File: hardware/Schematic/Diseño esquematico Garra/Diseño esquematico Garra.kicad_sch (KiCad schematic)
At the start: 12 parts, among them J1 Screw_Terminal_01x02

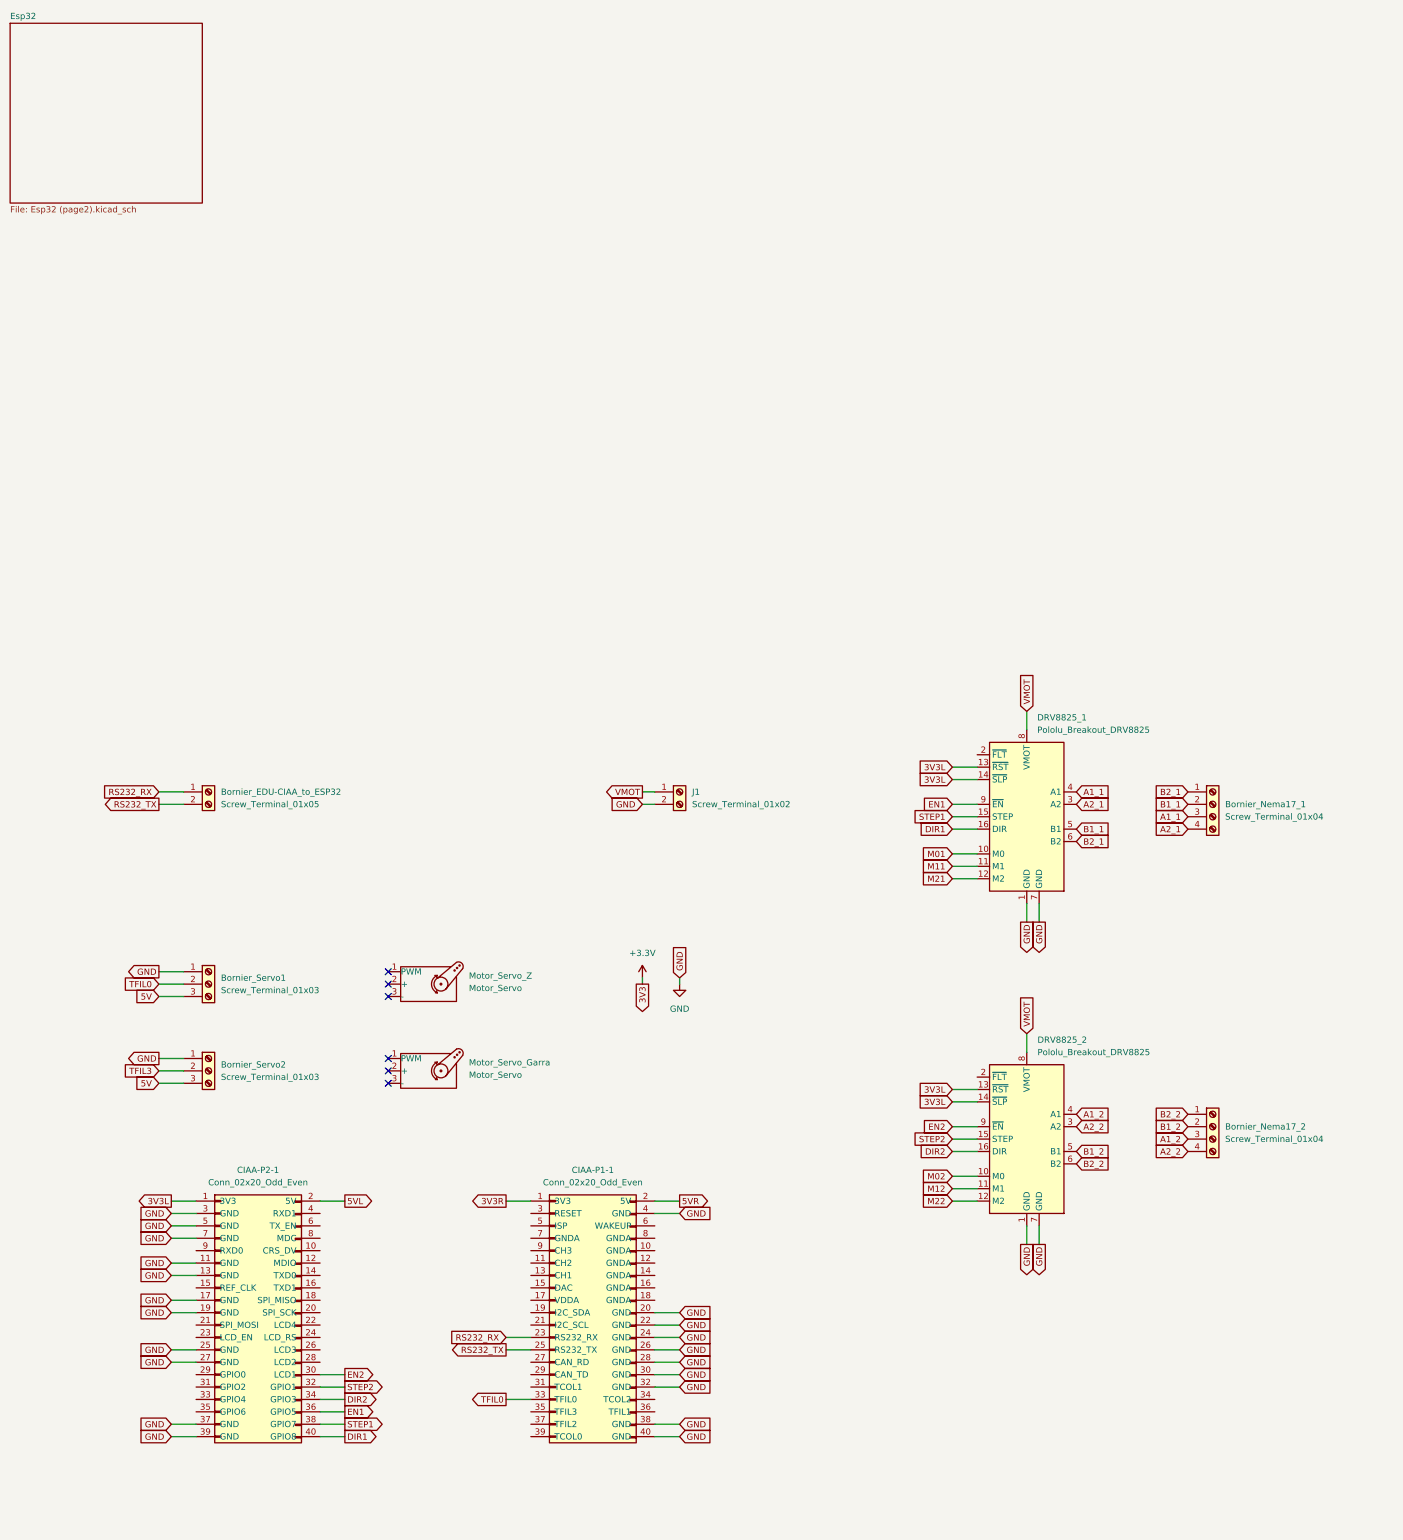
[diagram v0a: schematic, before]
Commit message: Schematics updated + PCB
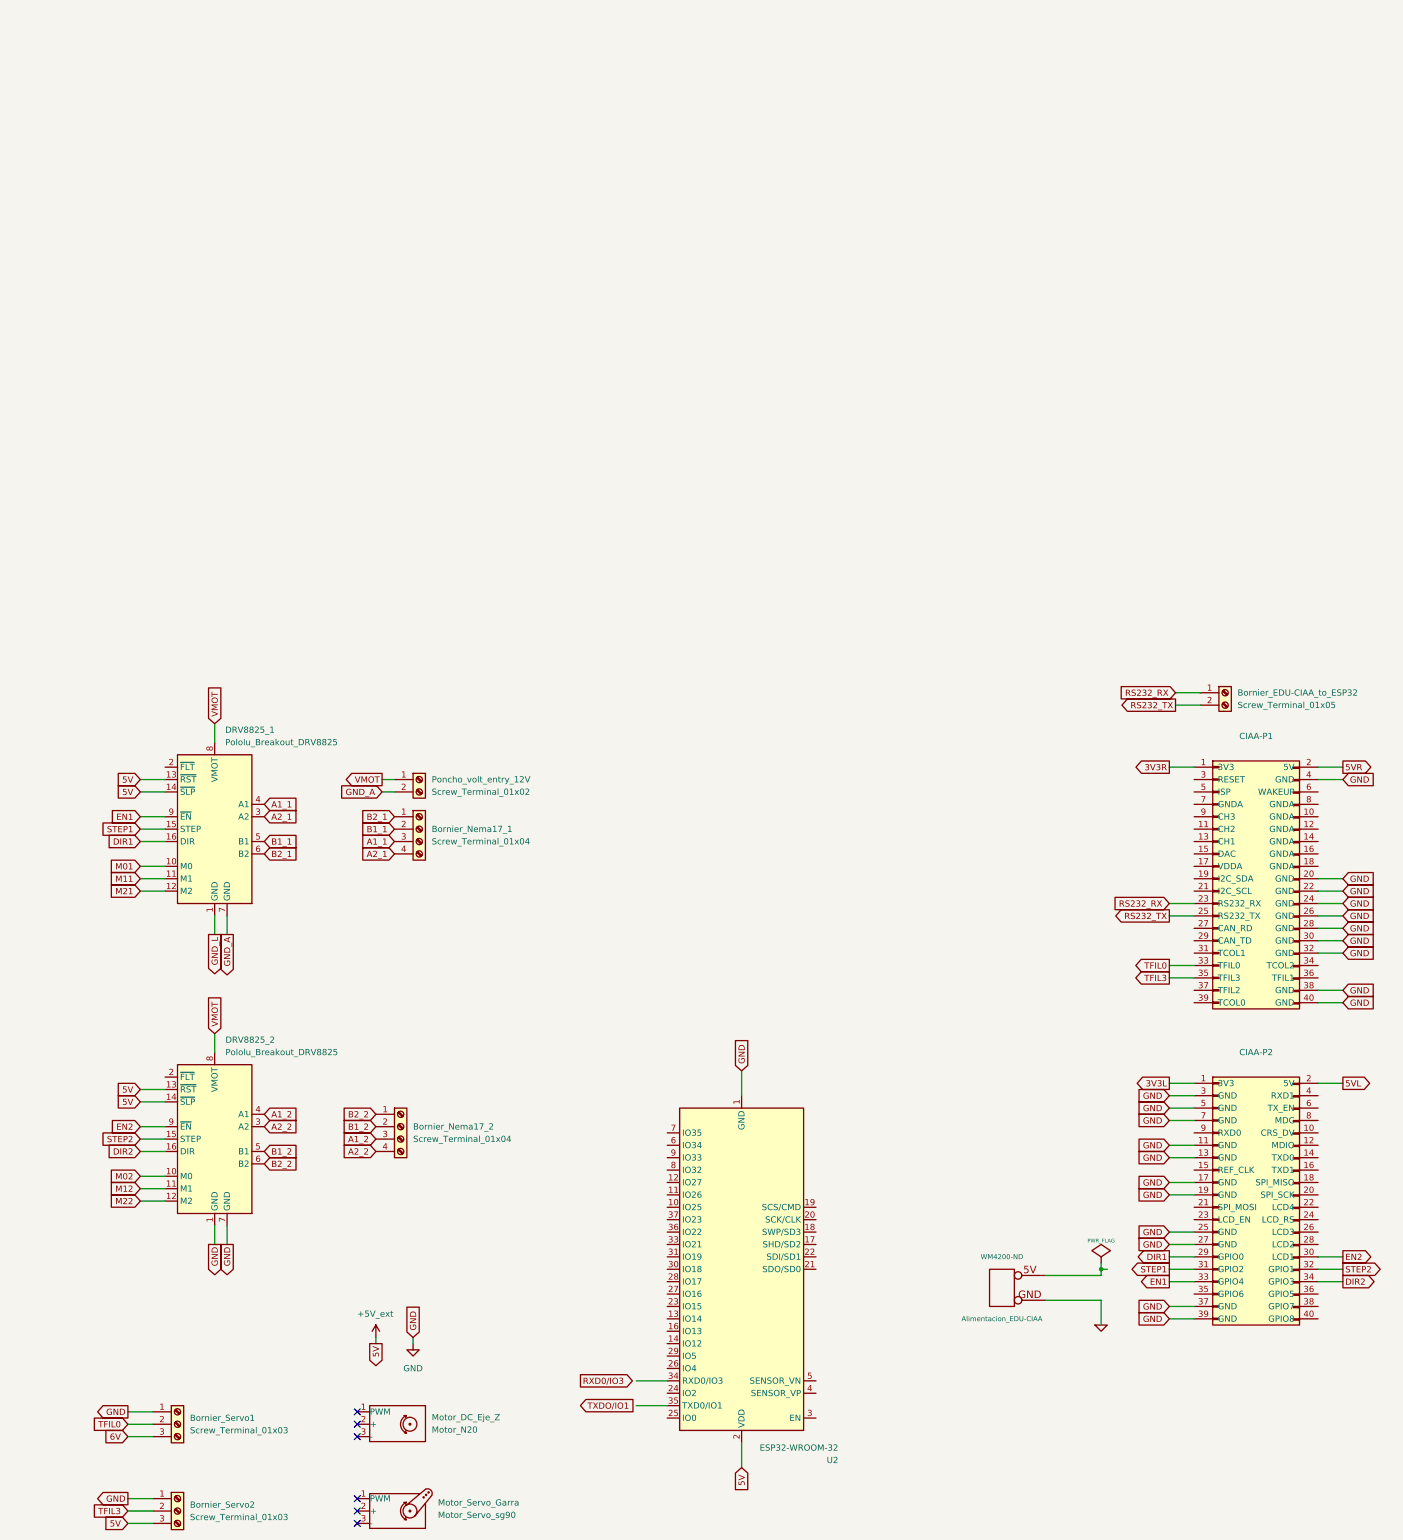
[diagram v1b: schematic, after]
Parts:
- added Alimentacion_EDU-CIAA: WM4200-ND, ~, symbol edu-ciaa-nxp:CONN_2
- added U2: ESP32-WROOM-32, RF_Module:ESP32-WROOM-32, symbol RF_Module:ESP32-WROOM-32
- CIAA-P1: renamed from CIAA-P1-1; value Conn_02x20_Odd_Even -> ~
- CIAA-P2: renamed from CIAA-P2-1; value Conn_02x20_Odd_Even -> ~
- Motor_DC_Eje_Z: renamed from Motor_Servo_Z; value Motor_Servo -> Motor_N20
- Motor_Servo_Garra: value Motor_Servo -> Motor_Servo_sg90
- renumbered J1 to Poncho_volt_entry_12V
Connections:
- net 3V3L: no longer DRV8825_1.13 (~{RST}), DRV8825_1.14 (~{SLP}), DRV8825_2.13 (~{RST}), DRV8825_2.14 (~{SLP})
- net DIR1: now also CIAA-P2.29 (GPIO0); no longer CIAA-P2.40 (GPIO8)
- net EN1: now also CIAA-P2.33 (GPIO4); no longer CIAA-P2.36 (GPIO5)
- net GND: now also Alimentacion_EDU-CIAA.GND (P1), U2.1 (GND), U2.15 (GND), U2.38 (GND), U2.39 (GND); no longer DRV8825_1.1 (GND), DRV8825_1.7 (GND), Poncho_volt_entry_12V.2 (Pin_2)
- net STEP1: now also CIAA-P2.31 (GPIO2); no longer CIAA-P2.38 (GPIO7)
- net TFIL3: now also CIAA-P1.35 (TFIL3)
- net 5V renamed +5V_ext
- net +5V_ext: now also DRV8825_1.13 (~{RST}), DRV8825_1.14 (~{SLP}), DRV8825_2.13 (~{RST}), DRV8825_2.14 (~{SLP}), U2.2 (VDD); no longer Bornier_Servo1.3 (Pin_3)
- new net 6V: Bornier_Servo1.3 (Pin_3)
- new net GND_A: DRV8825_1.7 (GND), Poncho_volt_entry_12V.2 (Pin_2)
- new net GND_L: DRV8825_1.1 (GND)
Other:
- removed sheet Esp32
- moved on the sheet: Bornier_EDU-CIAA_to_ESP32, Bornier_Nema17_1, Bornier_Nema17_2, Bornier_Servo1, Bornier_Servo2, CIAA-P1, CIAA-P2, DRV8825_1, DRV8825_2, Motor_Servo_Garra, Poncho_volt_entry_12V
